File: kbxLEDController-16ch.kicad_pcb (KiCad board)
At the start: 2 copper layers, 73 x 38.1 mm, 61 parts, among them J1 PWM_1-4, J2 PWM_5-8, J3 PWM_9-12, J4 PWM_13-16, J5 5 TO 24 VDC, J6 SERIAL+GPIO, Q1 PMV20ENR, Q10 PMV20ENR, Q11 PMV20ENR, Q12 PMV20ENR, Q13 PMV20ENR, Q14 PMV20ENR, Q15 PMV20ENR, Q16 PMV20ENR, Q2 PMV20ENR, Q3 PMV20ENR, Q4 PMV20ENR, Q5 PMV20ENR, Q6 PMV20ENR, Q7 PMV20ENR, Q8 PMV20ENR, Q9 PMV20ENR, SW1 RESET, SW2 BOOT/IO0, SW3 I34, SW4 I35, SW5 I36, SW6 I39, U1 ESP32-WROOM-32D, U2 AP2205-33Y, U3 TSOP382xx

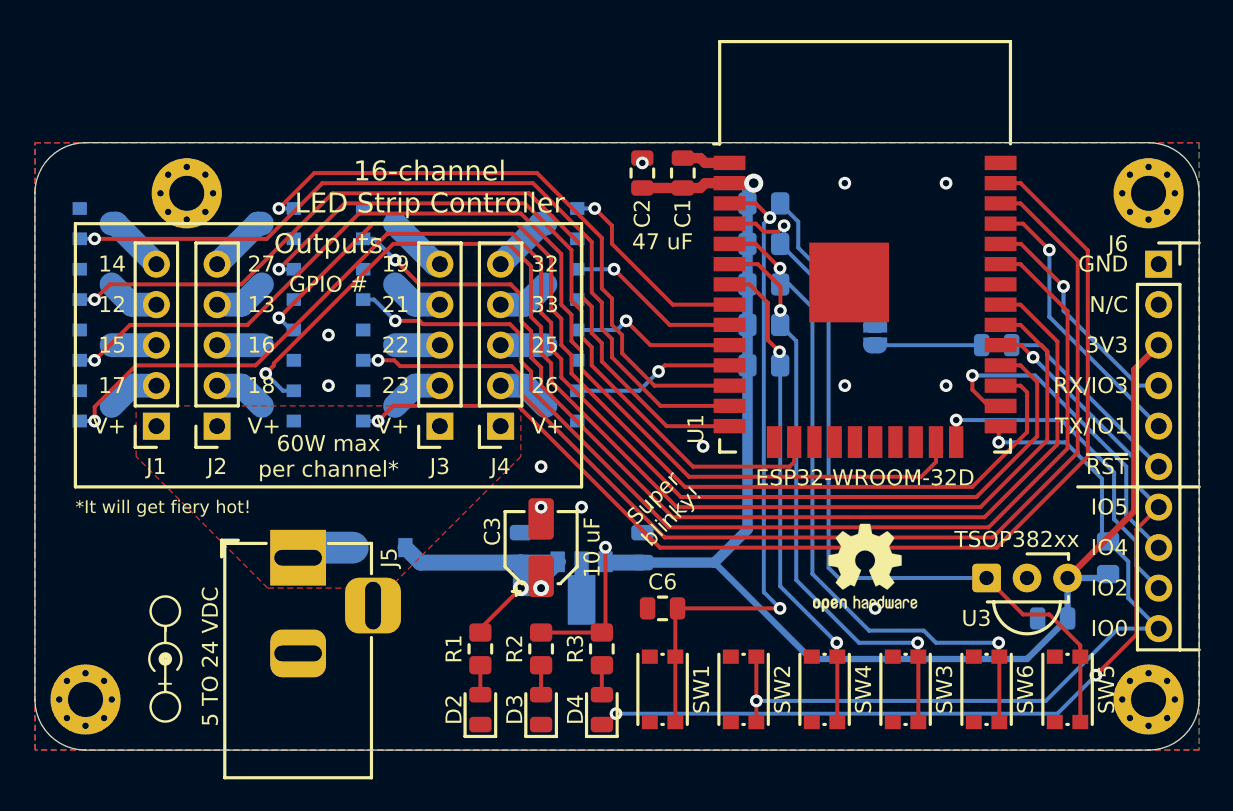
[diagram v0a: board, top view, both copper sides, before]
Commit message: v3
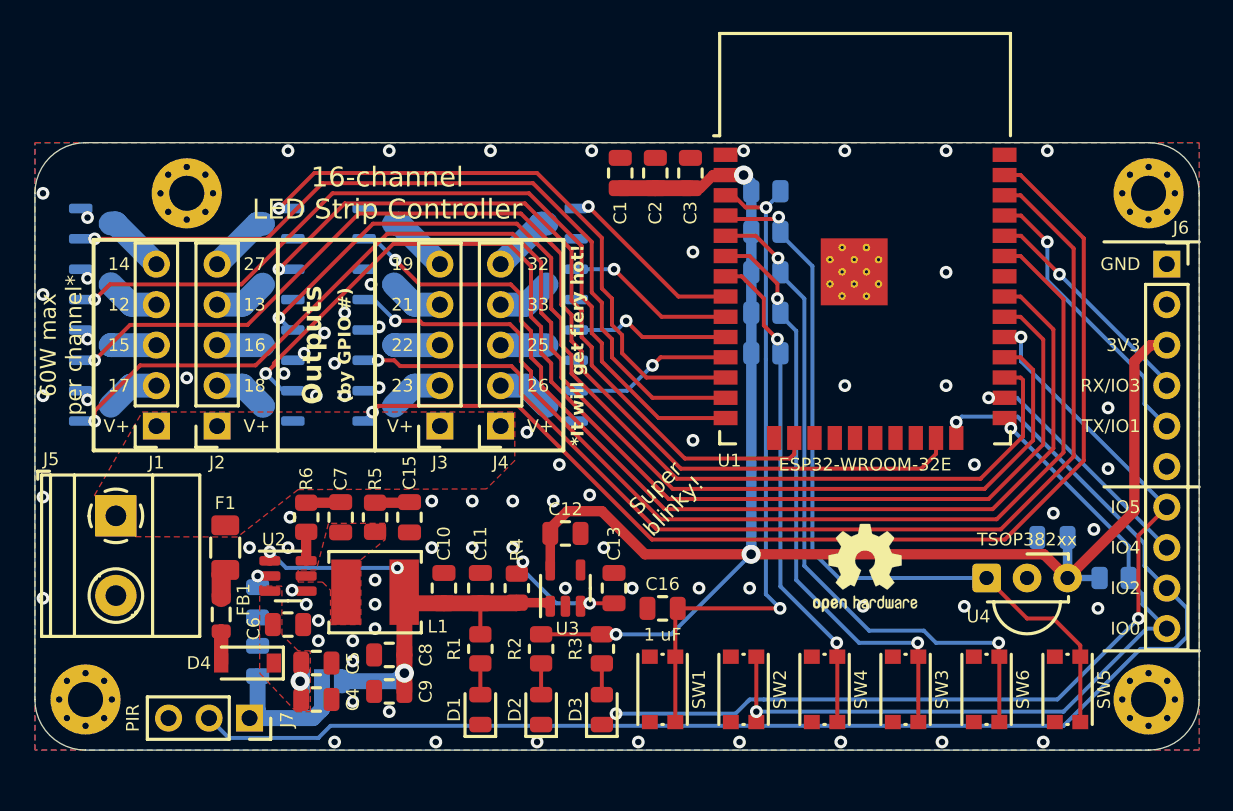
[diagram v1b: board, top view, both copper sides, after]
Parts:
- removed the REF** at (104.1, 106.7)
- added C10: 22 uF, Capacitor_SMD:C_0805_2012Metric, F.Cu at (121.5, 102.2)
- added C11: 1 uF, Capacitor_SMD:C_0805_2012Metric, F.Cu at (123.8, 102.2)
- added C12: 1 uF, Capacitor_SMD:C_0805_2012Metric, F.Cu at (129.2, 98.8)
- added C13: 10 uF, Capacitor_SMD:C_0805_2012Metric, F.Cu at (132.2, 102.2)
- added C14: 1 uF, Capacitor_SMD:C_0805_2012Metric, B.Cu at (109.9, 103.1)
- added C15: 100 pF, Capacitor_SMD:C_0805_2012Metric, F.Cu at (119.4, 97.8)
- added C18: 1 uF, Capacitor_SMD:C_0805_2012Metric, B.Cu at (109.9, 106.8)
- added C6: 100 nF, Capacitor_SMD:C_0805_2012Metric, F.Cu at (111.8, 104.5)
- added C8: 22 uF, Capacitor_SMD:C_0805_2012Metric, F.Cu at (118.1, 106.4)
- added C9: 22 uF, Capacitor_SMD:C_0805_2012Metric, F.Cu at (118.1, 108.7)
- added F1: 250 mA, Fuse:Fuse_1206_3216Metric, F.Cu at (107.8, 99.7)
- added FB1: 600R/1A, Inductor_SMD:L_0805_2012Metric, F.Cu at (107.6, 103.9)
- added J7: PIR, Connector_PinSocket_2.54mm:PinSocket_1x03_P2.54mm_Vertical, F.Cu at (109.3, 110.4)
- added L1: 6.8 uH, kbxLEDController-16ch:L_Murata_LQH5BPN_4.9x4.9mm, F.Cu at (117.2, 102.5)
- added QR*****: QR, kbxLEDController-16ch:QR, B.Cu at (155.4, 82.4)
- added R4: 100K, Resistor_SMD:R_0805_2012Metric, F.Cu at (126.1, 102.2)
- added R5: DNP, Resistor_SMD:R_0805_2012Metric, F.Cu at (117.2, 97.8)
- added R6: 0, Resistor_SMD:R_0805_2012Metric, F.Cu at (112.9, 97.8)
- added U3: AP2112K-3.3, Package_TO_SOT_SMD:SOT-23-5, F.Cu at (129.2, 102.2)
- C1: value 47 uF -> 10 uF
- C2: value 47 uF -> 1 uF
- C3: value 10 uF -> 100 nF; footprint Capacitor_SMD:CP_Elec_4x5.8 -> Capacitor_SMD:C_0805_2012Metric
- C4: value 1 uF -> 10 uF; moved to F.Cu
- C5: value 2.2 uF -> 1 uF; moved to F.Cu
- C7: moved to F.Cu
- D1: renamed from D2; value V_IN -> 5V
- D4: renamed from D1; moved to F.Cu
- J5: value 5 TO 24 VDC -> 6 TO 24 VDC; footprint Connector_BarrelJack:BarrelJack_Horizontal -> TerminalBlock_Phoenix:TerminalBlock_Phoenix_MKDS-1,5-2_1x02_P5.00mm_Horizontal
- JP1: value J7_~RST -> PIR_V+; footprint Jumper:SolderJumper-2_P1.3mm_Open_RoundedPad1.0x1.5mm -> Jumper:SolderJumper-3_P1.3mm_Open_RoundedPad1.0x1.5mm_NumberLabels
- R1: value 10K -> 8K2; footprint Resistor_SMD:R_0805_2012Metric_Pad1.15x1.40mm_HandSolder -> Resistor_SMD:R_0805_2012Metric
- R10: renamed from R7; footprint Resistor_SMD:R_0805_2012Metric_Pad1.15x1.40mm_HandSolder -> Resistor_SMD:R_0805_2012Metric
- R11: renamed from R8; footprint Resistor_SMD:R_0805_2012Metric_Pad1.15x1.40mm_HandSolder -> Resistor_SMD:R_0805_2012Metric
- R12: renamed from R9; footprint Resistor_SMD:R_0805_2012Metric_Pad1.15x1.40mm_HandSolder -> Resistor_SMD:R_0805_2012Metric
- R2, R3: value 1K6 -> 2K; footprint Resistor_SMD:R_0805_2012Metric_Pad1.15x1.40mm_HandSolder -> Resistor_SMD:R_0805_2012Metric
- R7: renamed from R4; footprint Resistor_SMD:R_0805_2012Metric_Pad1.15x1.40mm_HandSolder -> Resistor_SMD:R_0805_2012Metric
- R8: renamed from R5; footprint Resistor_SMD:R_0805_2012Metric_Pad1.15x1.40mm_HandSolder -> Resistor_SMD:R_0805_2012Metric
- R9: renamed from R6; footprint Resistor_SMD:R_0805_2012Metric_Pad1.15x1.40mm_HandSolder -> Resistor_SMD:R_0805_2012Metric
- U1: value ESP32-WROOM-32D -> ESP32-WROOM-32E
- U2: value AP2205-33Y -> AP63205WU; footprint Package_TO_SOT_SMD:SOT-89-3 -> Package_TO_SOT_SMD:TSOT-23-6; moved to F.Cu
- moved C7 42.5 mm to (115.1, 97.8), turned to -90 degrees
- moved JP1 40.9 mm to (113.9, 108.1), turned to 180 degrees
- moved REF** 37.0 mm to (124.6, 99.6)
- moved C3 25.3 mm to (137.0, 76.2), turned to -90 degrees
- moved C5 21.7 mm to (113.5, 106.9), turned to 180 degrees
- moved U2 18.4 mm to (111.8, 101.5), turned to 0 degrees
- moved C4 16.0 mm to (113.5, 109.2), turned to 180 degrees
- moved REF** 15.5 mm to (159.3, 93.5)
- moved J5 11.7 mm to (101.0, 97.7), turned to -90 degrees
- moved D4 11.0 mm to (109.2, 106.9)
- moved C17 5.08 mm to (159.7, 99.1)
- moved C1 3.93 mm to (132.6, 76.2), turned to -90 degrees
- moved R8 1.33 mm to (163.6, 101.6), turned to 0 degrees
- moved C2 0.81 mm to (134.8, 76.2), turned to -90 degrees
- moved R10 0.77 mm to (141.7, 87.5)
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- renumbered C6 to C16, C8 to C17, D3 to D2, D4 to D3, U3 to U4
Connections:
- C1 pad 1: +3V3 -> GND
- C1 pad 2: GND -> +3V3
- C16 pad 1: /~RESET -> /~{RESET}
- C2 pad 1: +3V3 -> GND
- C2 pad 2: GND -> +3V3
- C3 pad 1: Net-(C3-Pad1) -> GND
- C3 pad 2: GND -> +3V3
- C4 pad 1: Net-(C3-Pad1) -> GND
- C4 pad 2: GND -> +24V
- C5 pad 1: +3V3 -> GND
- C5 pad 2: GND -> +24V
- C7 pad 2: Net-(C7-Pad2) -> /SW
- D4 pad 1: Net-(C3-Pad1) -> +24V
- D4 pad 2: VDC -> Net-(D4-A)
- J6 pad 2: (no net) -> unconnected-(J6-Pin_2-Pad2)
- J6 pad 6: Net-(C7-Pad2) -> unconnected-(J6-Pin_6-Pad6)
- JP1 pad 1: /~RESET -> +5V
- JP1 pad 2: Net-(C7-Pad1) -> Net-(J7-Pin_1)
- R1 pad 1: Net-(C3-Pad1) -> +5V
- R7 pad 2: /~RESET -> /~{RESET}
- SW1 pad 1: /~RESET -> /~{RESET}
- U1 pad 17: (no net) -> unconnected-(U1-SHD/SD2-Pad17)
- U1 pad 18: (no net) -> unconnected-(U1-SWP/SD3-Pad18)
- U1 pad 19: (no net) -> unconnected-(U1-SCS/CMD-Pad19)
- U1 pad 20: (no net) -> unconnected-(U1-SCK/CLK-Pad20)
- U1 pad 21: (no net) -> unconnected-(U1-SDO/SD0-Pad21)
- U1 pad 22: (no net) -> unconnected-(U1-SDI/SD1-Pad22)
- U1 pad 3: /~RESET -> /~{RESET}
- U1 pad 32: (no net) -> unconnected-(U1-NC-Pad32)
- U2 pad 1: Net-(C3-Pad1) -> +5V
- U2 pad 2: GND -> Net-(U2-EN)
- U2 pad 3: +3V3 -> +24V
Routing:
- net /GPIO2: track 21.1 -> 86.7 mm
- net /~RESET: track 53.0 -> 0.00 mm, vias 2 -> 0
- net /~{RESET}: track 0.00 -> 43.4 mm, vias 0 -> 2
- net +5V: track 0.00 -> 30.8 mm, vias 0 -> 3
- net Net-(C3-Pad1): track 20.9 -> 0.00 mm, vias 2 -> 0
- net Net-(C7-Pad2): track 12.5 -> 0.00 mm
- net +3V3: track 96.8 -> 106.9 mm, vias 2 -> 3
- net Net-(J7-Pin_1): track 0.00 -> 9.37 mm
- net Net-(U3-EN): track 0.00 -> 8.64 mm, vias 0 -> 2
- net /GPIO4: track 21.0 -> 16.1 mm
- net Net-(C7-Pad1): track 6.69 -> 2.17 mm
- net VDC: track 3.69 -> 0.00 mm
- net GND: track 3.06 -> 0.00 mm, vias 12 -> 78
- net Net-(C15-Pad2): track 0.00 -> 2.17 mm
- net Net-(D4-A): track 0.00 -> 1.99 mm
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- added copper zone on F.Cu, net +24V
- added copper zone on F.Cu, net /SW
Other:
- net class Default removed
- net class Power3V3 removed
- net class PowerIn removed
- net class PowerLED removed
- net class PowerTerm removed
- board text added: "(by GPIO #)"
- board text added: "By @kbx81 https://github.com/kbx81 v3 — August 2023"
- board text added: "ESP32-powered 16-channel LED Strip Controller"
- board text added: "To use a 5 volt supply, short C14 to disable the buck converter, then bridge all three terminals of JP1."
- board text removed: "3V3 Regulation"
- board text removed: "By @kbx81 https://github.com/kbx81 v2 — October 2020"
- board text removed: "ESP32-powered LED Strip Controller"
- board text removed: "GPIO #"
